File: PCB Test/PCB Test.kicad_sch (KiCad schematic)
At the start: 47 parts, among them J1 Motor Terminal 2, J2 Conn_02x05_Odd_Even, J5 Motor Terminal 1, J6 Conn_02x03_Odd_Even, Q2 NMOS, Q3 NMOS, SW1 SW_Push, SW2 SW_Push, SW3 SW_Push, U1 ATmega4808-A, U2 TCRT5000, U3 TCRT5000, U4 TCRT5000, U5 MCP1700x-330xxTO

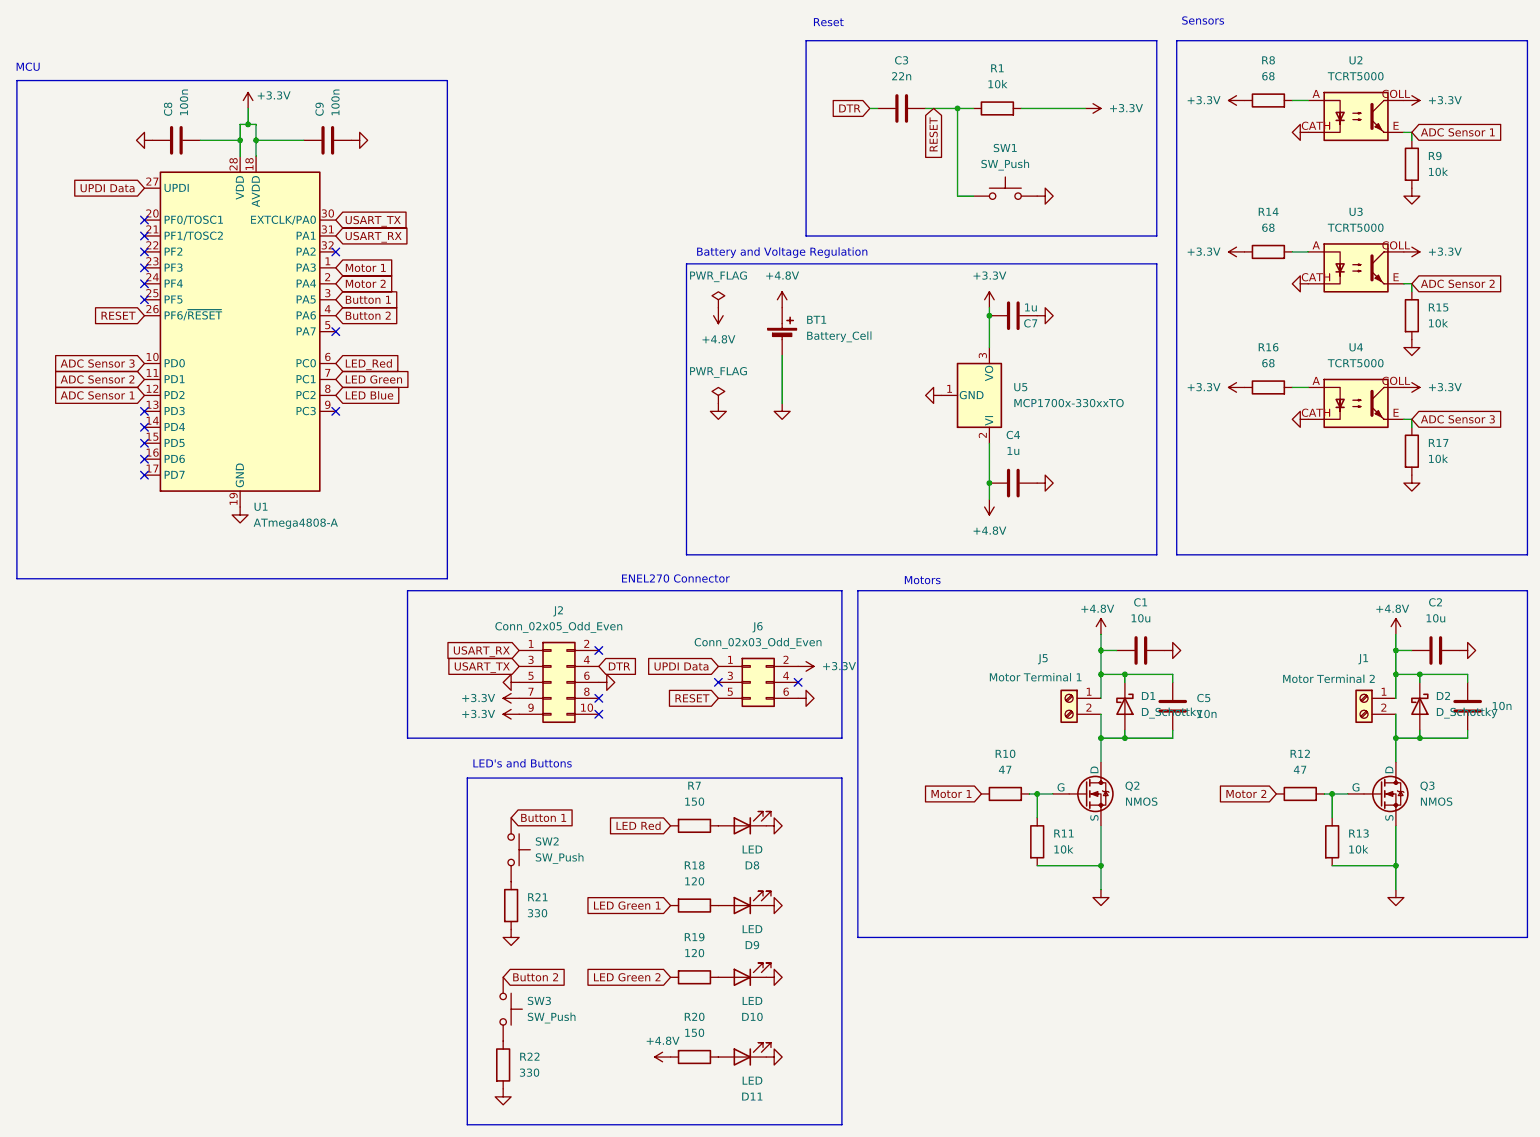
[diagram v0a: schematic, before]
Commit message: Final layout finished, moving on to motion transmition, need to extract gerber files
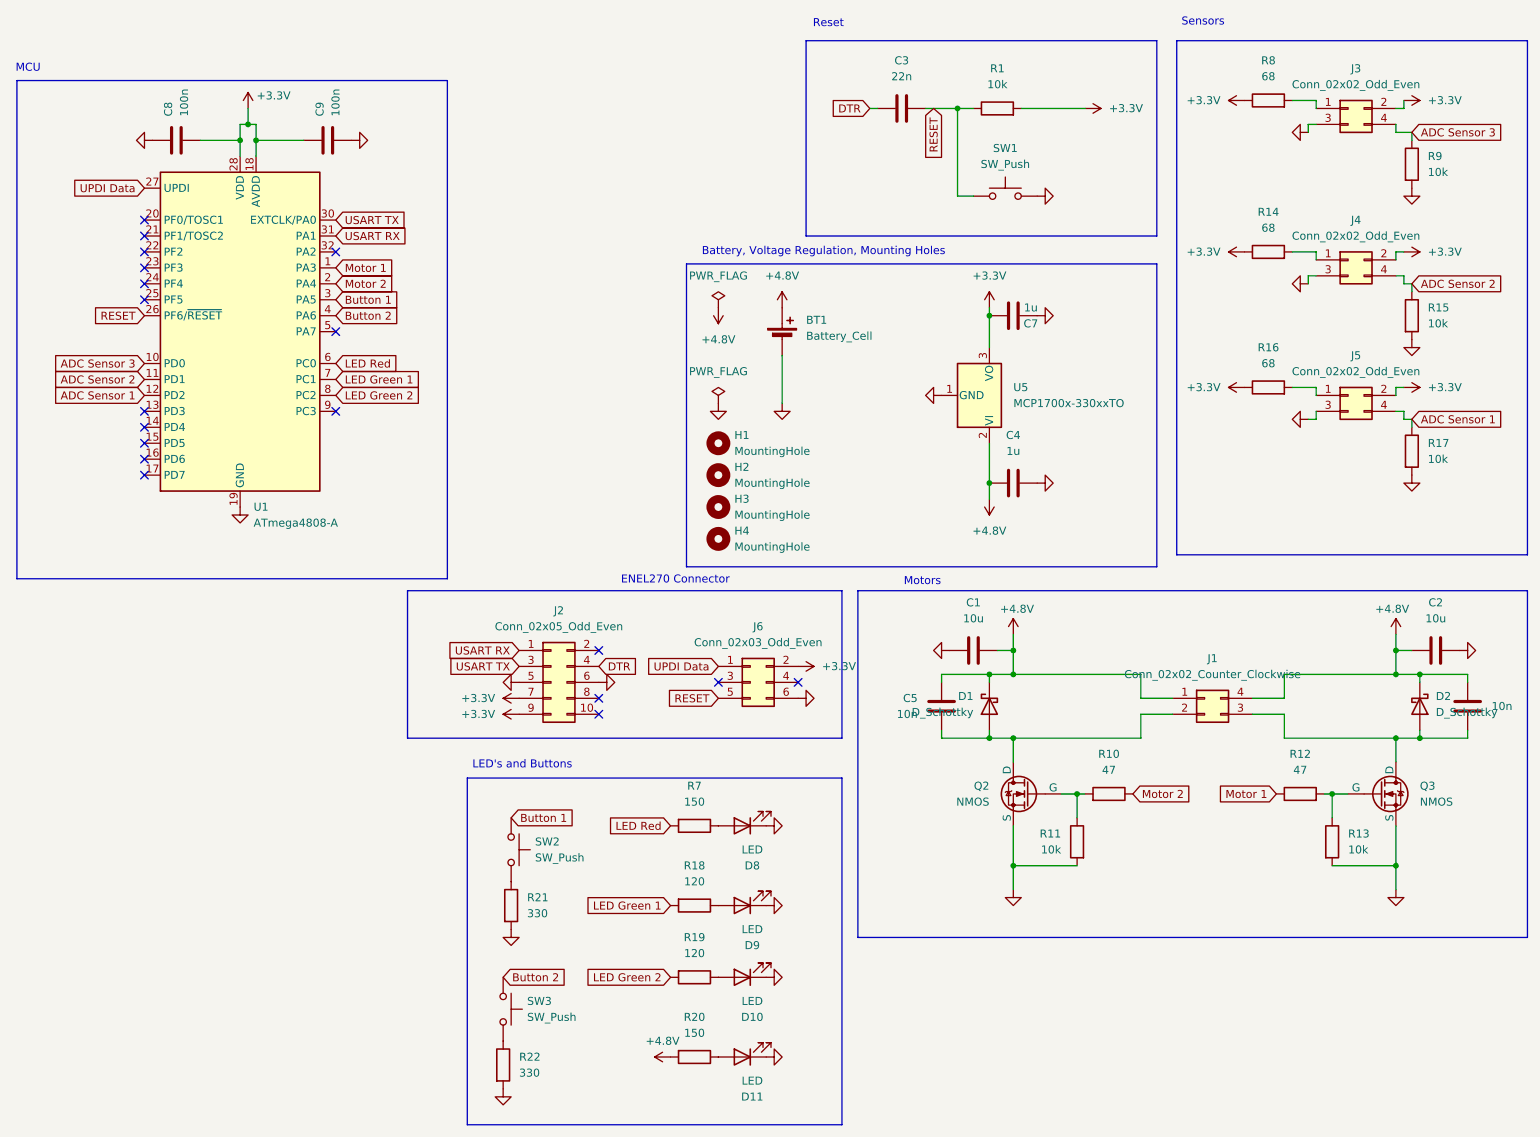
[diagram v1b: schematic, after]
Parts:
- removed J1: Motor Terminal 2, TerminalBlock:TerminalBlock_MaiXu_MX126-5.0-02P_1x02_P5.00mm, symbol Connector:Screw_Terminal_01x02
- removed J5: Motor Terminal 1, TerminalBlock:TerminalBlock_MaiXu_MX126-5.0-02P_1x02_P5.00mm, symbol Connector:Screw_Terminal_01x02
- removed U2, U3, U4: TCRT5000, Connector_Harwin:Harwin_LTek-Male_2x02_P2.00mm_Vertical, symbol tcrt5000:TCRT5000
- added H1, H2, H3, H4: MountingHole, MountingHole:MountingHole_2.2mm_M2, symbol Mechanical:MountingHole
- added J1: Conn_02x02_Counter_Clockwise, Connector:NS-Tech_Grove_1x04_P2mm_Vertical, symbol Connector_Generic:Conn_02x02_Counter_Clockwise
- added J3, J4, J5: Conn_02x02_Odd_Even, Connector_Harwin:Harwin_LTek-Male_2x02_P2.00mm_Vertical, symbol Connector_Generic:Conn_02x02_Odd_Even
- J2: footprint Connector_PinSocket_1.00mm:PinSocket_2x05_P1.00mm_Vertical_SMD -> Connector_PinHeader_1.00mm:PinHeader_2x05_P1.00mm_Vertical_SMD
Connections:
- net LED Blue is gone; now on net LED Green 2: U1.8 (PC2)
- net LED Green is gone; now on net LED Green 1: U1.7 (PC1)
- net LED_Red is gone; now on net LED Red: U1.6 (PC0)
- net +3.3V: now also J3.2 (Pin_2), J4.2 (Pin_2), J5.2 (Pin_2)
- net +4.8V: now also J1.1 (Pin_1), J1.4 (Pin_4)
- net ADC Sensor 1: now also R17.1, J5.4 (Pin_4); no longer R9.1
- net ADC Sensor 2: now also J4.4 (Pin_4)
- net ADC Sensor 3: now also R9.1, J3.4 (Pin_4); no longer R17.1
- net GND: now also J3.3 (Pin_3), J4.3 (Pin_3), J5.3 (Pin_3)
- net Motor 1: now also R12.1; no longer R10.1
- net Motor 2: now also R10.1; no longer R12.1
- net at C5.2, D1.2 (A), Q2.1 (D): now also J1.2 (Pin_2)
- net at R8.2: now also J3.1 (Pin_1)
- net at R14.2: now also J4.1 (Pin_1)
- net at C6.2, D2.2 (A), Q3.1 (D): now also J1.3 (Pin_3)
- net at R16.2: now also J5.1 (Pin_1)
- net USART_RX renamed USART RX
- net USART_TX renamed USART TX
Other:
- note added: "Battery, Voltage Regulation, Mounting Holes"
- note removed: "Battery and Voltage Regulation"
- moved on the sheet: C1, C5, D1, Q2, R10, R11
